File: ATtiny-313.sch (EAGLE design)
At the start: 13 parts

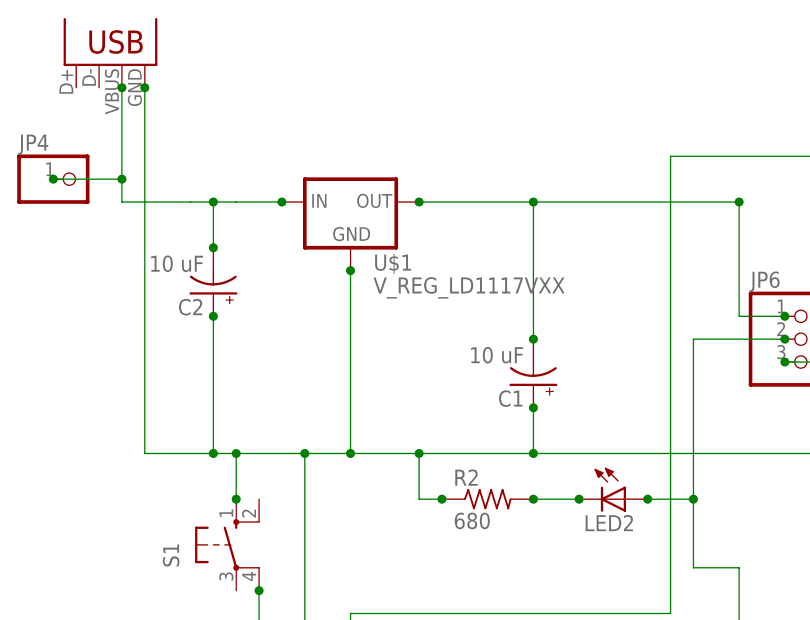
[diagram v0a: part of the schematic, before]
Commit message: more SMD goodness
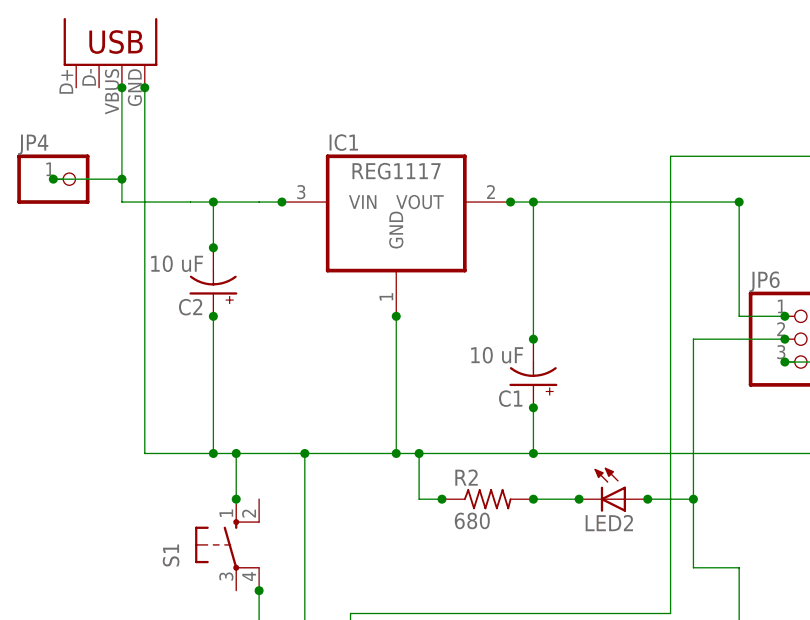
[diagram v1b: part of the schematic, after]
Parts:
- removed U$1: V_REG_LD1117VXX, SparkFun-PowerIC:V_REG_LD1117VXX
- added IC1: REG1117, burr-brown:REG1117
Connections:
- net N$1: now also IC1.VIN; no longer U$1.IN
- net N$3: now also IC1.GND; no longer U$1.GND
- net N$4: now also IC1.VOUT; no longer U$1.OUT
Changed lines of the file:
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@@
 <part name="ATTINY2313" library="ic-package" deviceset="DIL20" device="S"/>
 <part name="JP1" library="SparkFun-Connectors" deviceset="USB" device="PTH" value="USB-B"/>
-<part name="U$1" library="SparkFun-PowerIC" deviceset="V_REG_LD1117VXX" device=""/>
 <part name="C1" library="rcl" deviceset="CPOL-US" device="E1.8-4" value="10 uF"/>
 <part name="C2" library="rcl" deviceset="CPOL-US" device="E1.8-4" value="10 uF"/>
@@
 <part name="LED2" library="led" deviceset="LED" device="SMT1206"/>
 <part name="R2" library="resistor" deviceset="R-US_" device="R3216" value="680"/>
+<part name="IC1" library="burr-brown" deviceset="REG1117" device=""/>
 </parts>
 <sheets>
@@
 <instance part="ATTINY2313" gate="G$1" x="60.96" y="7.62"/>
 <instance part="JP1" gate="G$1" x="25.4" y="83.82" rot="R90"/>
-<instance part="U$1" gate="G$1" x="48.26" y="68.58"/>
 <instance part="C1" gate="G$1" x="68.58" y="48.26" rot="R180"/>
 <instance part="C2" gate="G$1" x="33.02" y="58.42" rot="R180"/>
@@
 <instance part="LED2" gate="G$1" x="78.74" y="35.56" rot="R270"/>
 <instance part="R2" gate="G$1" x="63.5" y="35.56"/>
+<instance part="IC1" gate="G$1" x="53.34" y="68.58"/>
 </instances>
 <busses>
@@
 <wire x1="22.86" y1="68.58" x2="30.48" y2="68.58" width="0.1524" layer="91"/>
 <wire x1="30.48" y1="68.58" x2="33.02" y2="68.58" width="0.1524" layer="91"/>
-<pinref part="U$1" gate="G$1" pin="IN"/>
-<wire x1="33.02" y1="68.58" x2="35.56" y2="68.58" width="0.1524" layer="91"/>
-<wire x1="35.56" y1="68.58" x2="40.64" y2="68.58" width="0.1524" layer="91"/>
+<wire x1="33.02" y1="68.58" x2="38.1" y2="68.58" width="0.1524" layer="91"/>
 <junction x="22.86" y="81.28"/>
-<junction x="40.64" y="68.58"/>
 <pinref part="C2" gate="G$1" pin="-"/>
 <wire x1="33.02" y1="63.5" x2="33.02" y2="68.58" width="0.1524" layer="91"/>
@@
 <junction x="22.86" y="71.12"/>
 <junction x="15.24" y="71.12"/>
+<pinref part="IC1" gate="G$1" pin="VIN"/>
+<wire x1="38.1" y1="68.58" x2="40.64" y2="68.58" width="0.1524" layer="91"/>
+<junction x="40.64" y="68.58"/>
 </segment>
 </net>
@@
 <wire x1="35.56" y1="40.64" x2="43.18" y2="40.64" width="0.1524" layer="91"/>
 <wire x1="43.18" y1="40.64" x2="48.26" y2="40.64" width="0.1524" layer="91"/>
-<wire x1="48.26" y1="40.64" x2="55.88" y2="40.64" width="0.1524" layer="91"/>
+<wire x1="48.26" y1="40.64" x2="53.34" y2="40.64" width="0.1524" layer="91"/>
+<wire x1="53.34" y1="40.64" x2="55.88" y2="40.64" width="0.1524" layer="91"/>
 <wire x1="55.88" y1="40.64" x2="68.58" y2="40.64" width="0.1524" layer="91"/>
 <wire x1="68.58" y1="40.64" x2="68.58" y2="45.72" width="0.1524" layer="91"/>
-<pinref part="U$1" gate="G$1" pin="GND"/>
-<wire x1="48.26" y1="60.96" x2="48.26" y2="40.64" width="0.1524" layer="91"/>
-<junction x="48.26" y="60.96"/>
-<junction x="48.26" y="40.64"/>
 <junction x="68.58" y="45.72"/>
 <junction x="33.02" y="55.88"/>
@@
 <pinref part="R2" gate="G$1" pin="1"/>
 <junction x="58.42" y="35.56"/>
+<pinref part="IC1" gate="G$1" pin="GND"/>
+<wire x1="53.34" y1="55.88" x2="53.34" y2="40.64" width="0.1524" layer="91"/>
+<junction x="53.34" y="40.64"/>
+<junction x="53.34" y="55.88"/>
 </segment>
 </net>
@@
 <segment>
 <pinref part="C1" gate="G$1" pin="-"/>
-<pinref part="U$1" gate="G$1" pin="OUT"/>
-<junction x="55.88" y="68.58"/>
-<wire x1="55.88" y1="68.58" x2="68.58" y2="68.58" width="0.1524" layer="91"/>
 <wire x1="68.58" y1="68.58" x2="91.44" y2="68.58" width="0.1524" layer="91"/>
-<junction x="68.58" y="68.58"/>
 <wire x1="68.58" y1="68.58" x2="68.58" y2="53.34" width="0.1524" layer="91"/>
 <junction x="68.58" y="53.34"/>
@@
 <junction x="96.52" y="55.88"/>
 <junction x="91.44" y="68.58"/>
-</segment>
-</net>
+<pinref part="IC1" gate="G$1" pin="VOUT"/>
+<wire x1="68.58" y1="68.58" x2="66.04" y2="68.58" width="0.1524" layer="91"/>
+<junction x="68.58" y="68.58"/>
+<junction x="66.04" y="68.58"/>
+</segment>
+</net>

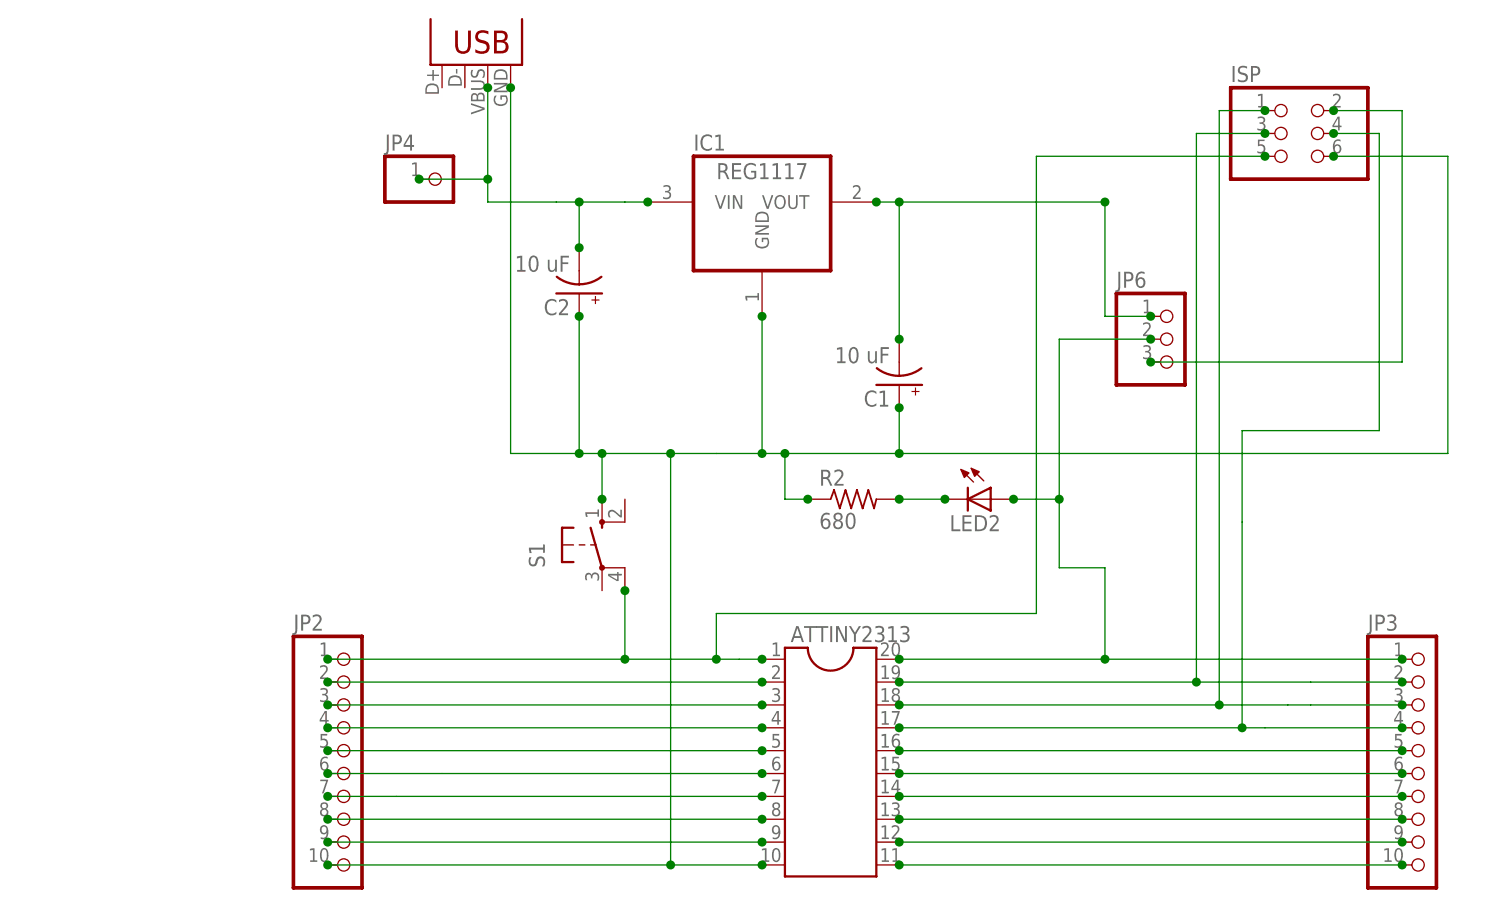
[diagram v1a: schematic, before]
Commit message: tightened up the design
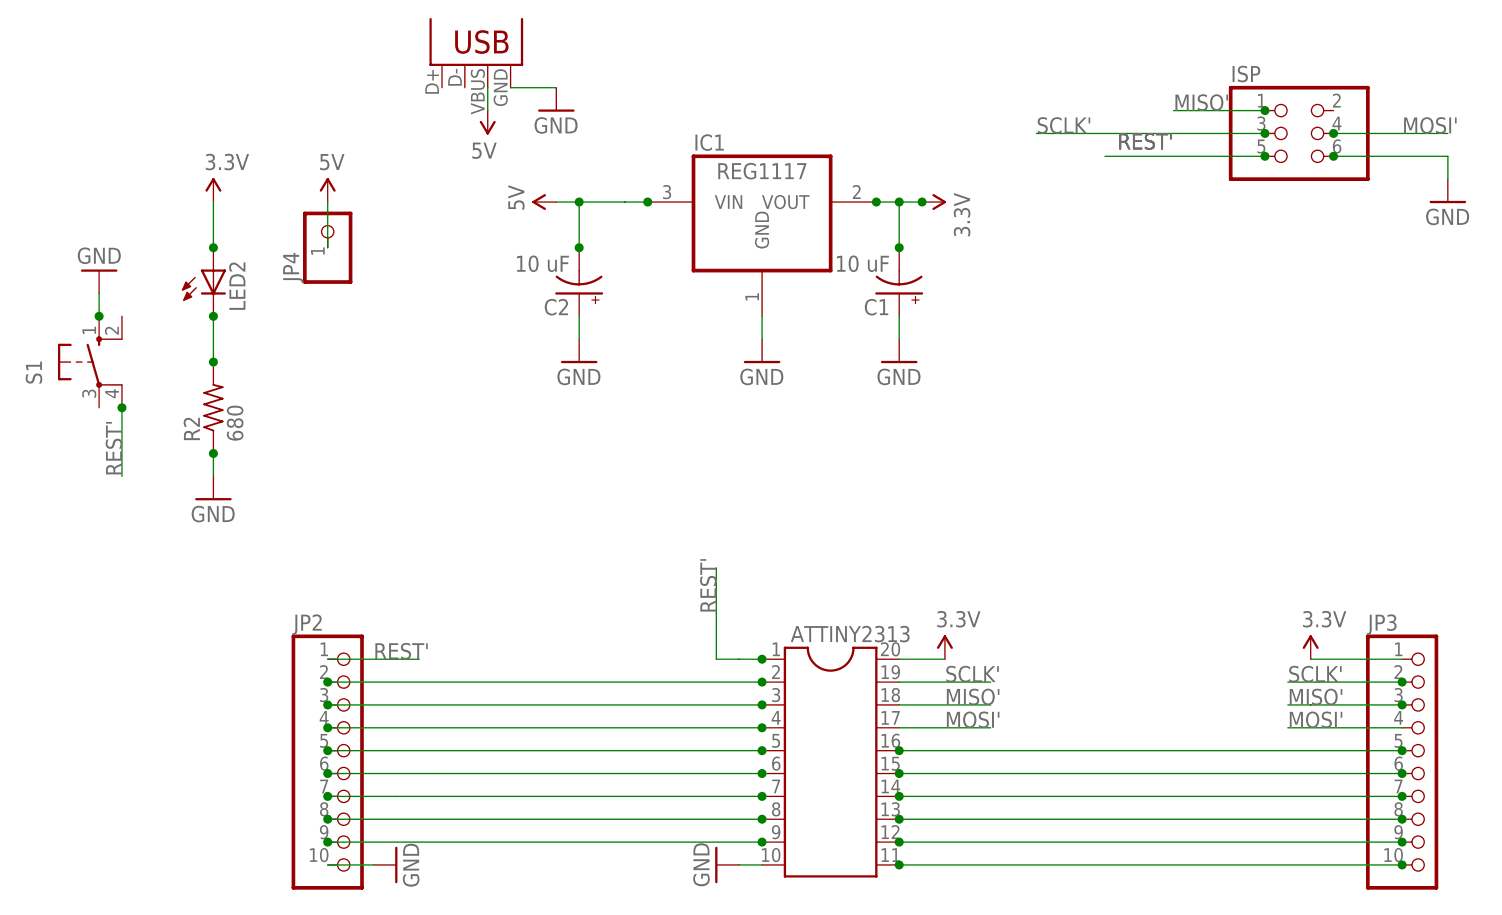
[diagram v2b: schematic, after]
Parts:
- removed JP6: (no value), pinhead:PINHD-1X3
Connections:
- net ISP renamed MISO'
- net N$1 renamed 5V
- net N$14 renamed SCLK'
- net N$16 renamed MOSI'
- net N$3 renamed GND
- net N$5 renamed REST'
- removed net N$2: ATTINY2313.20, JP3.1, JP6.2, LED2.A
- removed net N$23: ISP.2, JP6.3
- removed net N$4: C1.-, IC1.VOUT, JP6.1
- new net 3.3V: ATTINY2313.20, C1.-, IC1.VOUT, JP3.1, LED2.A
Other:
- note added: "MISO'"
- note added: "MOSI'"
- note added: "REST'"
- note added: "SCLK'"
- moved on the sheet: C1, JP4, LED2, R2, S1
